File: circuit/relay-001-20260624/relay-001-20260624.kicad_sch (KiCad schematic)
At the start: 15 parts, among them J1 Dribbler_{Back}, J10 Conn_01x02_Pin, J11 Motor1, J12 Motor2, J13 Motor3, J14 Motor4, J15 Conn_01x02_Pin, J2 Kicker-Board, J3 MD-Board, J4 Main-Board, J5 Linesensor_{Power}, J6 Conn_01x02_Pin, J7 Conn_01x02_Pin, J8 Linesensor_{Power}, J9 Linesensor_{UART}

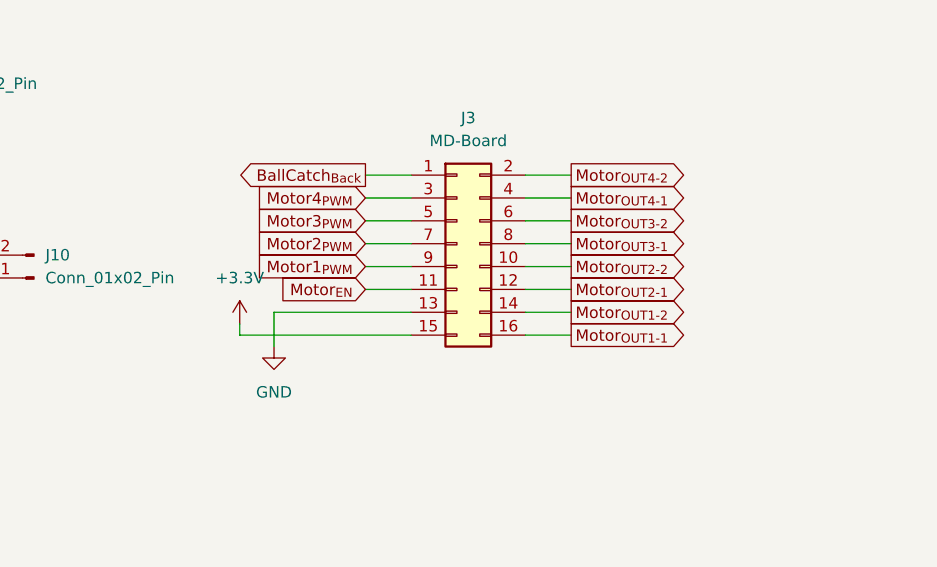
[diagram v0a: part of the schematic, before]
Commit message: Update 供給基板のボード図を更新
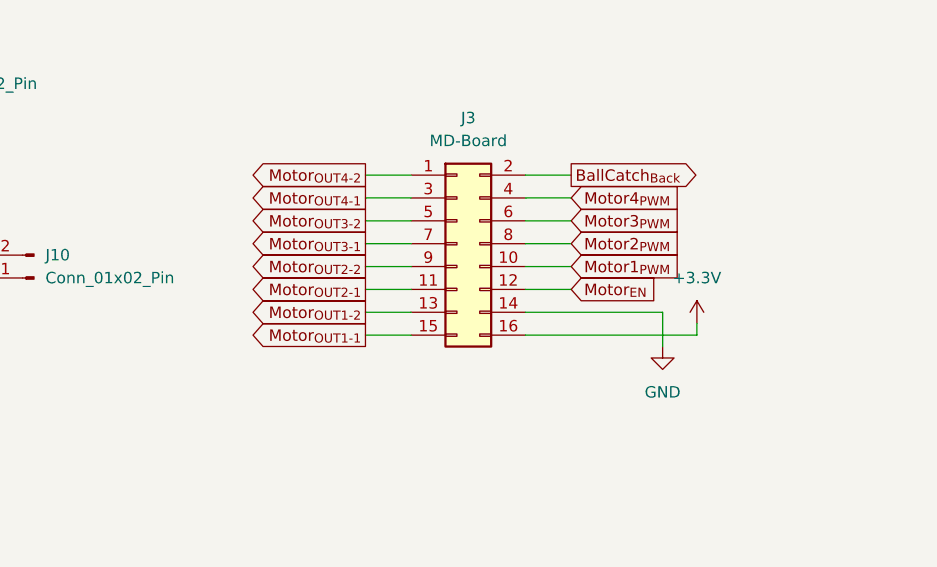
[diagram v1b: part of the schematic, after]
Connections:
- net +3.3V: now also J3.16 (Pin_16); no longer J3.15 (Pin_15)
- net BallCatch_{Back}: now also J3.2 (Pin_2); no longer J3.1 (Pin_1)
- net GND: now also J3.14 (Pin_14); no longer J3.13 (Pin_13)
- net Motor1_{PWM}: now also J3.10 (Pin_10); no longer J3.9 (Pin_9)
- net Motor2_{PWM}: now also J3.8 (Pin_8); no longer J3.7 (Pin_7)
- net Motor3_{PWM}: now also J3.6 (Pin_6); no longer J3.5 (Pin_5)
- net Motor4_{PWM}: now also J3.4 (Pin_4); no longer J3.3 (Pin_3)
- net Motor_{EN}: now also J3.12 (Pin_12); no longer J3.11 (Pin_11)
- net Motor_{OUT1-1}: now also J3.15 (Pin_15); no longer J3.16 (Pin_16)
- net Motor_{OUT1-2}: now also J3.13 (Pin_13); no longer J3.14 (Pin_14)
- net Motor_{OUT2-1}: now also J3.11 (Pin_11); no longer J3.12 (Pin_12)
- net Motor_{OUT2-2}: now also J3.9 (Pin_9); no longer J3.10 (Pin_10)
- net Motor_{OUT3-1}: now also J3.7 (Pin_7); no longer J3.8 (Pin_8)
- net Motor_{OUT3-2}: now also J3.5 (Pin_5); no longer J3.6 (Pin_6)
- net Motor_{OUT4-1}: now also J3.3 (Pin_3); no longer J3.4 (Pin_4)
- net Motor_{OUT4-2}: now also J3.1 (Pin_1); no longer J3.2 (Pin_2)
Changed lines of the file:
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@@
 	(wire
 		(pts
-			(xy 185.42 148.59) (xy 180.34 148.59)
+			(xy 167.64 148.59) (xy 162.56 148.59)
 		)
 		(stroke
@@
 	(wire
 		(pts
-			(xy 148.59 149.86) (xy 148.59 151.13)
+			(xy 199.39 149.86) (xy 199.39 151.13)
 		)
 		(stroke
@@
 	(wire
 		(pts
-			(xy 148.59 151.13) (xy 167.64 151.13)
+			(xy 180.34 151.13) (xy 199.39 151.13)
 		)
 		(stroke
@@
 	(wire
 		(pts
-			(xy 152.4 148.59) (xy 167.64 148.59)
+			(xy 180.34 148.59) (xy 195.58 148.59)
 		)
 		(stroke
@@
 	(wire
 		(pts
-			(xy 152.4 148.59) (xy 152.4 152.4)
+			(xy 195.58 148.59) (xy 195.58 152.4)
 		)
 		(stroke
@@
 	(wire
 		(pts
-			(xy 185.42 151.13) (xy 180.34 151.13)
+			(xy 167.64 151.13) (xy 162.56 151.13)
 		)
 		(stroke
@@
 	(global_label "Motor3_{PWM}"
 		(shape input)
-		(at 162.56 138.43 180)
+		(at 185.42 138.43 0)
 		(fields_autoplaced yes)
 		(effects
@@
 				(size 1.27 1.27)
 			)
-			(justify right)
+			(justify left)
 		)
 		(property "Intersheetrefs" "${INTERSHEET_REFS}"
-			(at 151.4905 138.43 0)
+			(at 196.4895 138.43 0)
 			(hide yes)
 			(show_name no)
@@
 					(size 1.27 1.27)
 				)
-				(justify right)
+				(justify left)
 			)
 		)
@@
 	(global_label "Motor_{OUT4-1}"
 		(shape output)
-		(at 185.42 135.89 0)
+		(at 162.56 135.89 180)
 		(fields_autoplaced yes)
 		(effects
@@
 				(size 1.27 1.27)
 			)
-			(justify left)
+			(justify right)
 		)
 		(property "Intersheetrefs" "${INTERSHEET_REFS}"
-			(at 196.7687 135.89 0)
+			(at 151.2113 135.89 0)
 			(hide yes)
 			(show_name no)
@@
 					(size 1.27 1.27)
 				)
-				(justify left)
+				(justify right)
 			)
 		)
@@
 	(global_label "Motor_{EN}"
 		(shape input)
-		(at 162.56 146.05 180)
+		(at 185.42 146.05 0)
 		(fields_autoplaced yes)
 		(effects
@@
 				(size 1.27 1.27)
 			)
-			(justify right)
+			(justify left)
 		)
 		(property "Intersheetrefs" "${INTERSHEET_REFS}"
-			(at 153.6767 146.05 0)
+			(at 194.3033 146.05 0)
 			(hide yes)
 			(show_name no)
@@
 					(size 1.27 1.27)
 				)
-				(justify right)
+				(justify left)
 			)
 		)
@@
 	(global_label "Motor_{OUT2-2}"
 		(shape output)
-		(at 185.42 143.51 0)
+		(at 162.56 143.51 180)
 		(fields_autoplaced yes)
 		(effects
@@
 				(size 1.27 1.27)
 			)
-			(justify left)
+			(justify right)
 		)
 		(property "Intersheetrefs" "${INTERSHEET_REFS}"
-			(at 196.7687 143.51 0)
+			(at 151.2113 143.51 0)
 			(hide yes)
 			(show_name no)
@@
 					(size 1.27 1.27)
 				)
-				(justify left)
+				(justify right)
 			)
 		)
@@
 	(global_label "Motor2_{PWM}"
 		(shape input)
-		(at 162.56 140.97 180)
+		(at 185.42 140.97 0)
 		(fields_autoplaced yes)
 		(effects
@@
 				(size 1.27 1.27)
 			)
-			(justify right)
+			(justify left)
 		)
 		(property "Intersheetrefs" "${INTERSHEET_REFS}"
-			(at 151.4905 140.97 0)
+			(at 196.4895 140.97 0)
 			(hide yes)
 			(show_name no)
@@
 					(size 1.27 1.27)
 				)
-				(justify right)
+				(justify left)
 			)
 		)
@@
 	(global_label "Motor1_{PWM}"
 		(shape input)
-		(at 162.56 143.51 180)
+		(at 185.42 143.51 0)
 		(fields_autoplaced yes)
 		(effects
@@
 				(size 1.27 1.27)
 			)
-			(justify right)
+			(justify left)
 		)
 		(property "Intersheetrefs" "${INTERSHEET_REFS}"
-			(at 151.4905 143.51 0)
+			(at 196.4895 143.51 0)
 			(hide yes)
 			(show_name no)
@@
 					(size 1.27 1.27)
 				)
-				(justify right)
+				(justify left)
 			)
 		)
@@
 	(global_label "Motor4_{PWM}"
 		(shape input)
-		(at 162.56 135.89 180)
+		(at 185.42 135.89 0)
 		(fields_autoplaced yes)
 		(effects
@@
 				(size 1.27 1.27)
 			)
-			(justify right)
+			(justify left)
 		)
 		(property "Intersheetrefs" "${INTERSHEET_REFS}"
-			(at 151.4905 135.89 0)
+			(at 196.4895 135.89 0)
 			(hide yes)
 			(show_name no)
@@
 					(size 1.27 1.27)
 				)
-				(justify right)
+				(justify left)
 			)
 		)
@@
 	(global_label "Motor_{OUT1-2}"
 		(shape output)
-		(at 185.42 148.59 0)
+		(at 162.56 148.59 180)
 		(fields_autoplaced yes)
 		(effects
@@
 				(size 1.27 1.27)
 			)
-			(justify left)
+			(justify right)
 		)
 		(property "Intersheetrefs" "${INTERSHEET_REFS}"
-			(at 196.7687 148.59 0)
+			(at 151.2113 148.59 0)
 			(hide yes)
 			(show_name no)
@@
 					(size 1.27 1.27)
 				)
-				(justify left)
+				(justify right)
 			)
 		)
@@
 	(global_label "Motor_{OUT2-1}"
 		(shape output)
-		(at 185.42 146.05 0)
+		(at 162.56 146.05 180)
 		(fields_autoplaced yes)
 		(effects
@@
 				(size 1.27 1.27)
 			)
-			(justify left)
+			(justify right)
 		)
 		(property "Intersheetrefs" "${INTERSHEET_REFS}"
-			(at 196.7687 146.05 0)
+			(at 151.2113 146.05 0)
 			(hide yes)
 			(show_name no)
@@
 					(size 1.27 1.27)
 				)
-				(justify left)
+				(justify right)
 			)
 		)
@@
 	(global_label "Motor_{OUT1-1}"
 		(shape output)
-		(at 185.42 151.13 0)
+		(at 162.56 151.13 180)
 		(fields_autoplaced yes)
 		(effects
@@
 				(size 1.27 1.27)
 			)
-			(justify left)
+			(justify right)
 		)
 		(property "Intersheetrefs" "${INTERSHEET_REFS}"
-			(at 196.7687 151.13 0)
+			(at 151.2113 151.13 0)
 			(hide yes)
 			(show_name no)
@@
 					(size 1.27 1.27)
 				)
-				(justify left)
+				(justify right)
 			)
 		)
@@
 	(global_label "BallCatch_{Back}"
 		(shape output)
-		(at 162.56 133.35 180)
+		(at 185.42 133.35 0)
 		(fields_autoplaced yes)
 		(effects
@@
 				(size 1.27 1.27)
 			)
-			(justify right)
+			(justify left)
 		)
 		(property "Intersheetrefs" "${INTERSHEET_REFS}"
-			(at 149.6678 133.35 0)
+			(at 198.3122 133.35 0)
 			(hide yes)
 			(show_name no)
@@
 					(size 1.27 1.27)
 				)
-				(justify right)
+				(justify left)
 			)
 		)
@@
 	(global_label "Motor_{OUT3-2}"
 		(shape output)
-		(at 185.42 138.43 0)
+		(at 162.56 138.43 180)
 		(fields_autoplaced yes)
 		(effects
@@
 				(size 1.27 1.27)
 			)
-			(justify left)
+			(justify right)
 		)
 		(property "Intersheetrefs" "${INTERSHEET_REFS}"
-			(at 196.7687 138.43 0)
+			(at 151.2113 138.43 0)
 			(hide yes)
 			(show_name no)
@@
 					(size 1.27 1.27)
 				)
-				(justify left)
+				(justify right)
 			)
 		)
@@
 	(global_label "Motor_{OUT3-1}"
 		(shape output)
-		(at 185.42 140.97 0)
+		(at 162.56 140.97 180)
 		(fields_autoplaced yes)
 		(effects
@@
 				(size 1.27 1.27)
 			)
-			(justify left)
+			(justify right)
 		)
 		(property "Intersheetrefs" "${INTERSHEET_REFS}"
-			(at 196.7687 140.97 0)
+			(at 151.2113 140.97 0)
 			(hide yes)
 			(show_name no)
@@
 					(size 1.27 1.27)
 				)
-				(justify left)
+				(justify right)
 			)
 		)
@@
 	(global_label "Motor_{OUT4-2}"
 		(shape output)
-		(at 185.42 133.35 0)
+		(at 162.56 133.35 180)
 		(fields_autoplaced yes)
 		(effects
@@
 				(size 1.27 1.27)
 			)
-			(justify left)
+			(justify right)
 		)
 		(property "Intersheetrefs" "${INTERSHEET_REFS}"
-			(at 196.7687 133.35 0)
+			(at 151.2113 133.35 0)
 			(hide yes)
 			(show_name no)
@@
 					(size 1.27 1.27)
 				)
-				(justify left)
+				(justify right)
 			)
 		)
@@
 	(symbol
 		(lib_id "power:GND")
-		(at 152.4 152.4 0)
+		(at 195.58 152.4 0)
 		(unit 1)
 		(body_style 1)
@@
 		(fields_autoplaced yes)
 		(property "Reference" "#PWR08"
-			(at 152.4 158.75 0)
+			(at 195.58 158.75 0)
 			(hide yes)
 			(show_name no)
@@
 		)
 		(property "Value" "GND"
-			(at 152.4 157.48 0)
+			(at 195.58 157.48 0)
 			(show_name no)
 			(do_not_autoplace no)
@@
 		)
 		(property "Footprint" ""
-			(at 152.4 152.4 0)
+			(at 195.58 152.4 0)
 			(hide yes)
 			(show_name no)
@@
 		)
 		(property "Datasheet" ""
-			(at 152.4 152.4 0)
+			(at 195.58 152.4 0)
 			(hide yes)
 			(show_name no)
@@
 		)
 		(property "Description" "Power symbol creates a global label with name \"GND\" , ground"
-			(at 152.4 152.4 0)
+			(at 195.58 152.4 0)
 			(hide yes)
 			(show_name no)
@@
 	(symbol
 		(lib_id "power:+3.3V")
-		(at 148.59 149.86 0)
+		(at 199.39 149.86 0)
 		(unit 1)
 		(body_style 1)
@@
 		(fields_autoplaced yes)
 		(property "Reference" "#PWR07"
-			(at 148.59 153.67 0)
+			(at 199.39 153.67 0)
 			(hide yes)
 			(show_name no)
@@
 		)
 		(property "Value" "+3.3V"
-			(at 148.59 144.78 0)
+			(at 199.39 144.78 0)
 			(show_name no)
 			(do_not_autoplace no)
@@
 		)
 		(property "Footprint" ""
-			(at 148.59 149.86 0)
+			(at 199.39 149.86 0)
 			(hide yes)
 			(show_name no)
@@
 		)
 		(property "Datasheet" ""
-			(at 148.59 149.86 0)
+			(at 199.39 149.86 0)
 			(hide yes)
 			(show_name no)
@@
 		)
 		(property "Description" "Power symbol creates a global label with name \"+3.3V\""
-			(at 148.59 149.86 0)
+			(at 199.39 149.86 0)
 			(hide yes)
 			(show_name no)

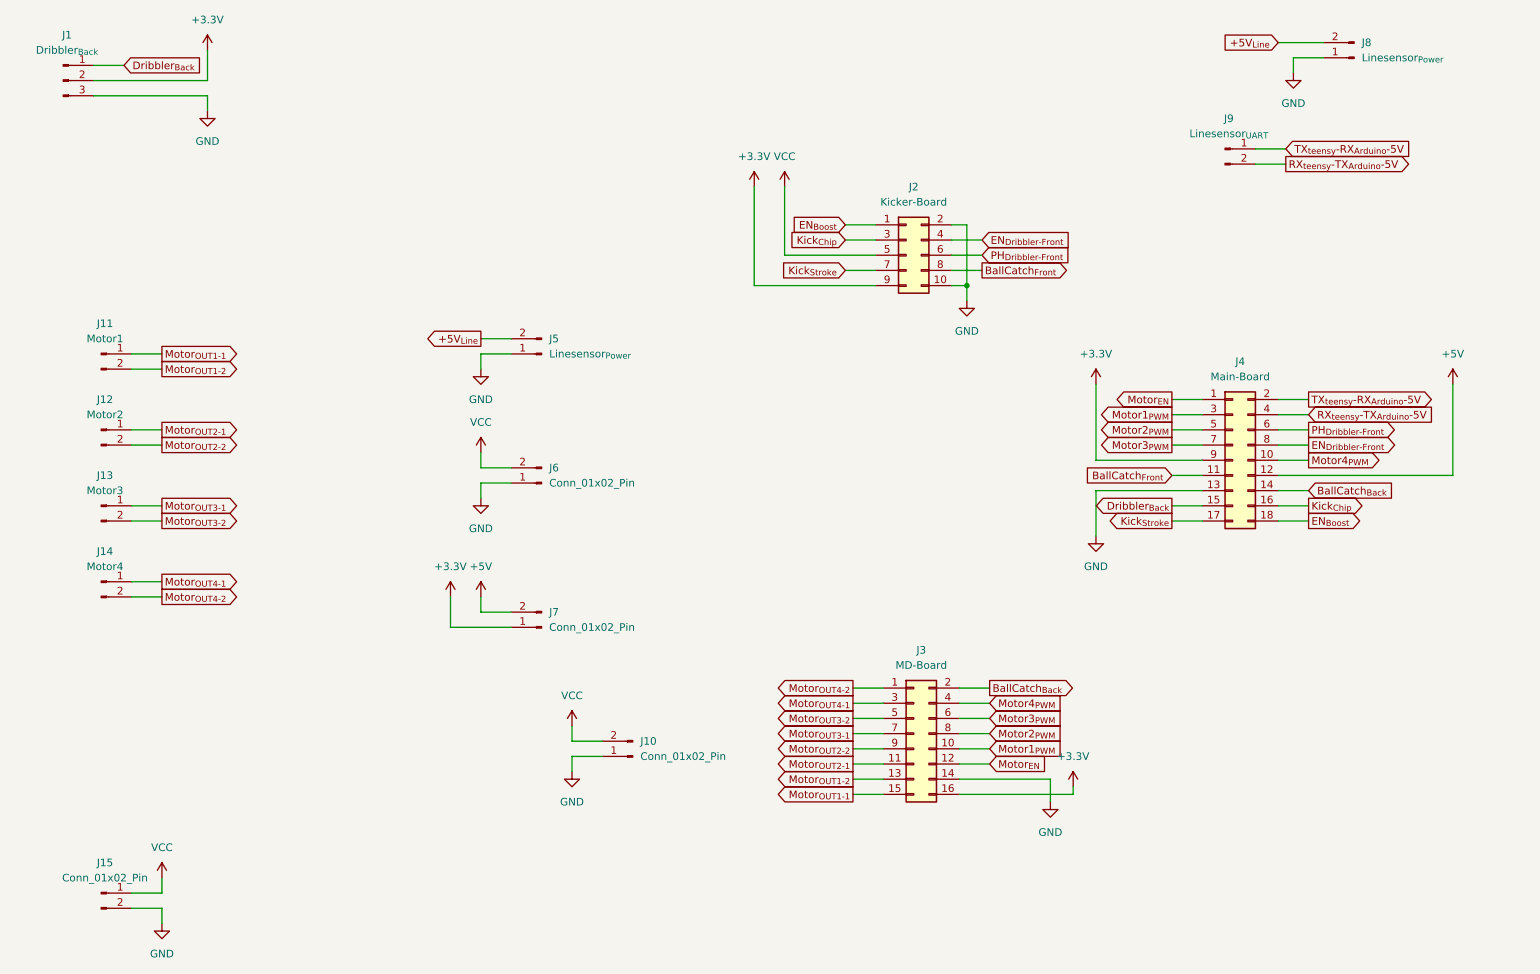
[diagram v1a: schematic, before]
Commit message: Update 供給基板のボード図の修正とDR完了、再DR求
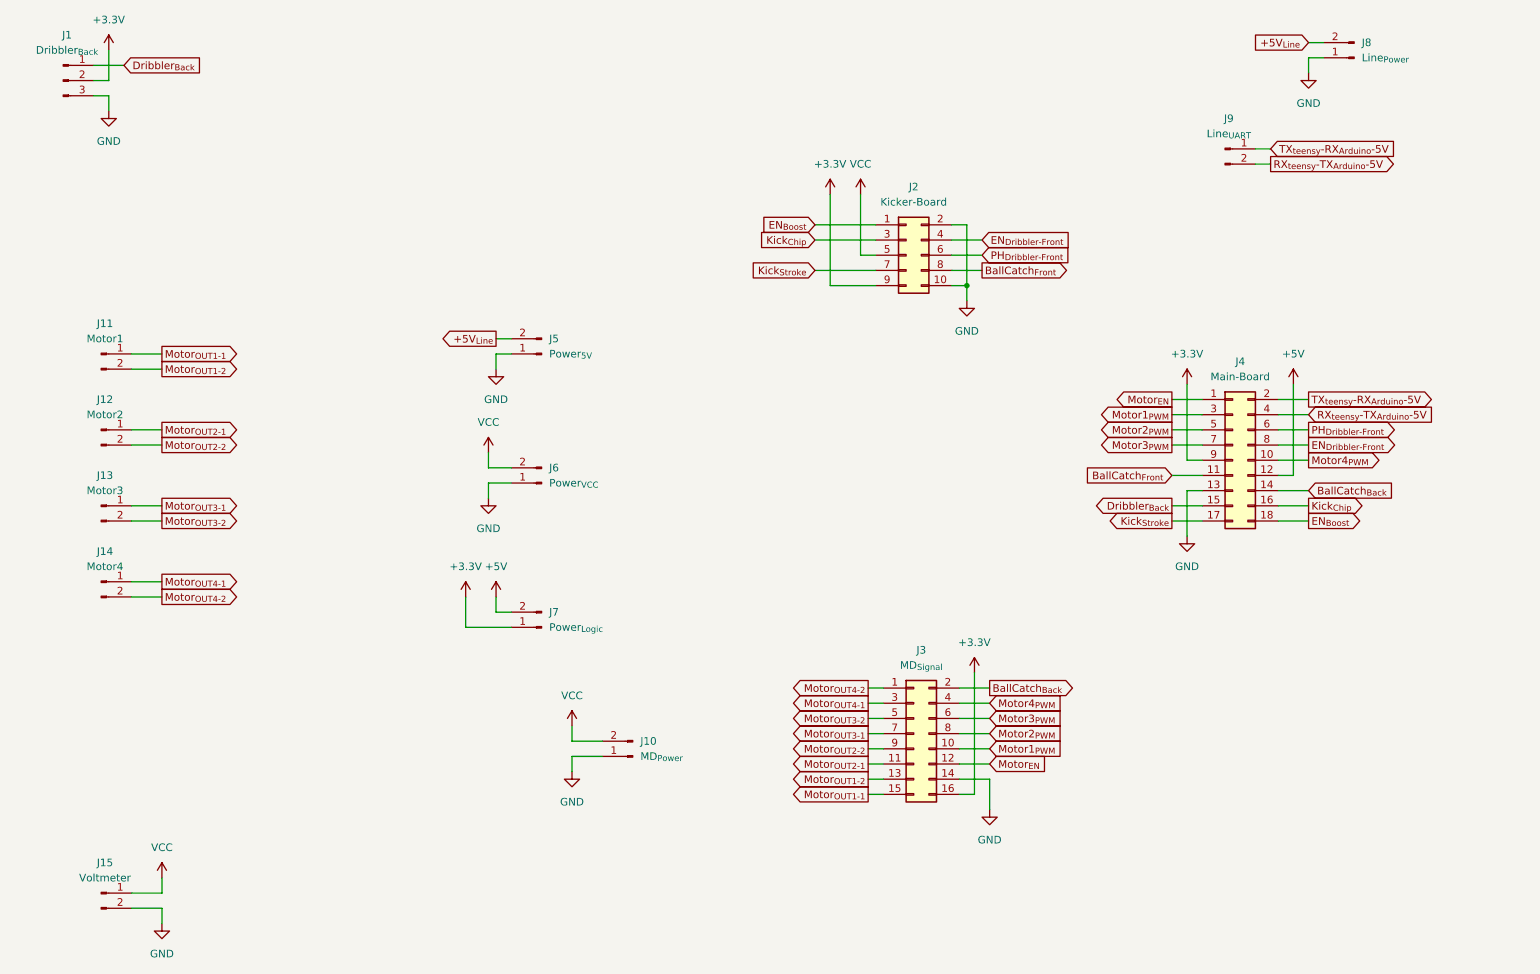
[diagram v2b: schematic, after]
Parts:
- J10: value Conn_01x02_Pin -> MD_{Power}
- J15: value Conn_01x02_Pin -> Voltmeter
- J3: value MD-Board -> MD_{Signal}
- J5: value Linesensor_{Power} -> Power_{5V}
- J6: value Conn_01x02_Pin -> Power_{VCC}
- J7: value Conn_01x02_Pin -> Power_{Logic}
- J8: value Linesensor_{Power} -> Line_{Power}
- J9: value Linesensor_{UART} -> Line_{UART}
